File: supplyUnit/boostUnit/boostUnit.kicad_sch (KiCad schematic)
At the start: 25 parts, among them J1 Conn_02x03_Counter_Clockwise, J2 Conn_02x03_Counter_Clockwise

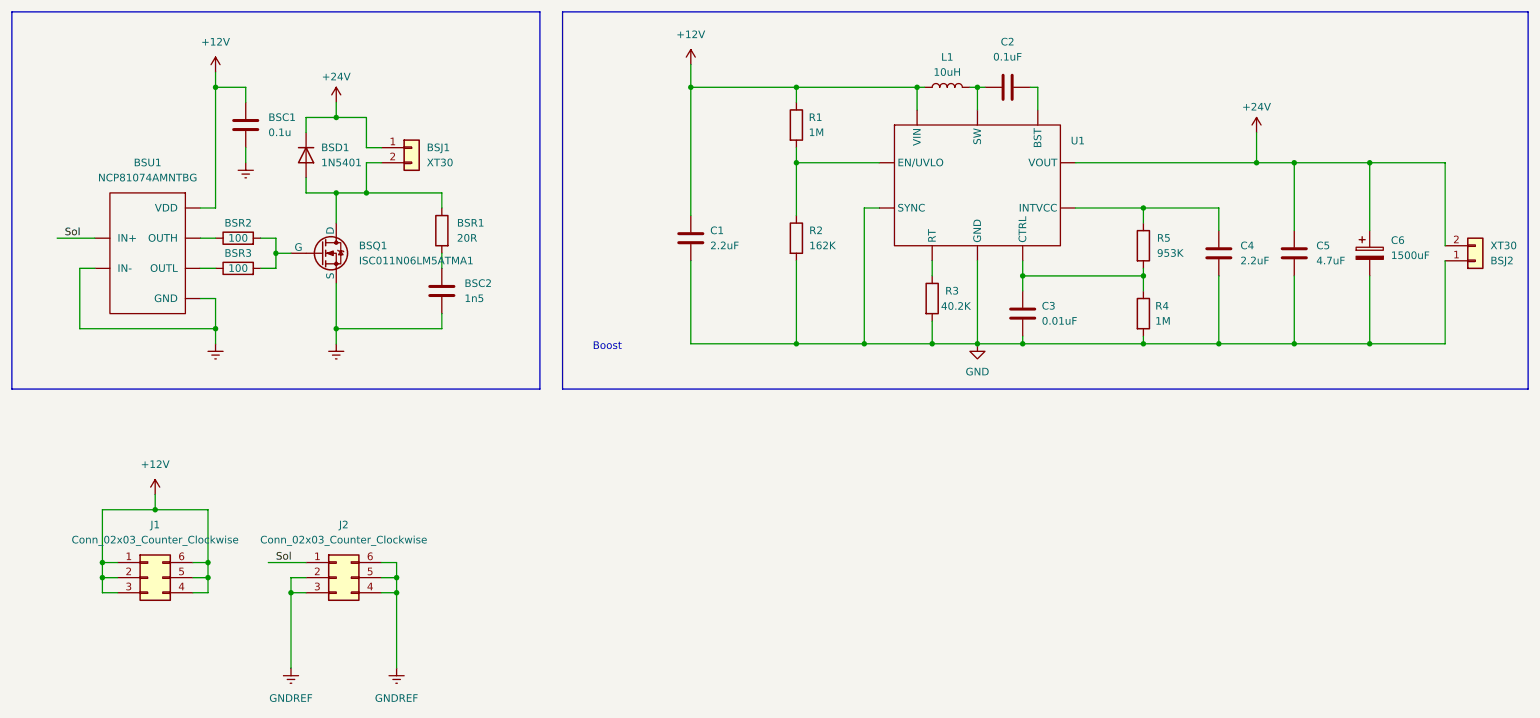
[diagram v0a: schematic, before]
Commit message: Revert
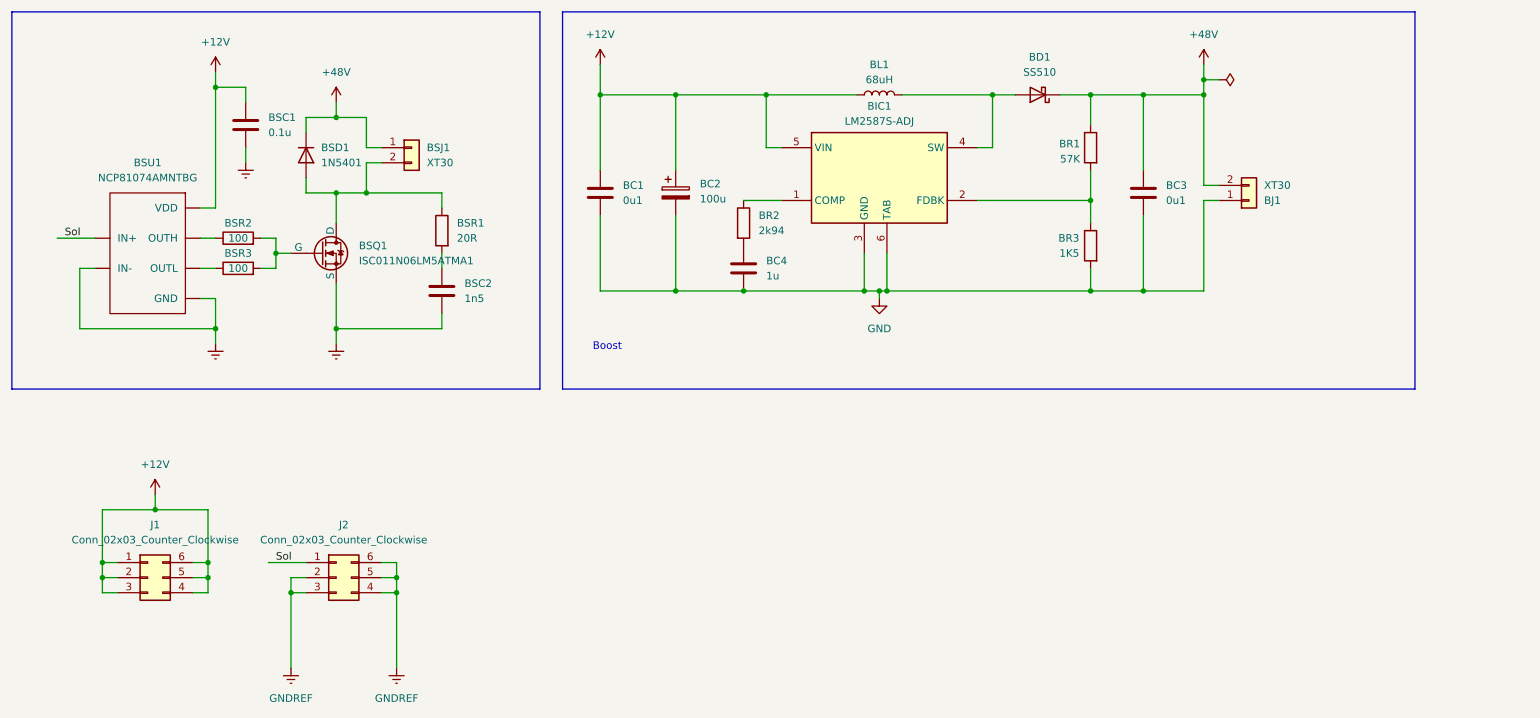
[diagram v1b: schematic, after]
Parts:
- removed BSJ2: XT30, Library:AMASS_XT30PW-F_1x02_P2.50mm_Horizontal, symbol Connector_Generic:Conn_01x02
- removed C1, C4: 2.2uF, Boost:cap0805, symbol Device:C
- removed C2: 0.1uF, Boost:cap0402, symbol Device:C
- removed C3: 0.01uF, Boost:cap0402, symbol Device:C
- removed C5: 4.7uF, Boost:res0805, symbol Device:C
- removed C6: 1500uF, Boost:CP_Radial_D16.0mm_P7.50mm, symbol Device:C_Polarized
- removed L1: 10uH, Boost:res0805, symbol Device:L
- removed R1, R4: 1M, Boost:res0402, symbol Device:R
- removed R2: 162K, Boost:res0402, symbol Device:R
- removed R3: 40.2K, Boost:res0402, symbol Device:R
- removed R5: 953K, Boost:res0402, symbol Device:R
- removed U1: ~, Boost:LT8338, symbol boostUnit:LT8338
- added BC1, BC3: 0u1, Library:cap0603, symbol Device:C
- added BC2: 100u, Capacitor_SMD:CP_Elec_8x6.5, symbol Device:C_Polarized
- added BC4: 1u, Library:cap0603, symbol Device:C
- added BD1: SS510, Library:SMA (DO-214AC), symbol Device:D_Schottky
- added BIC1: LM2587S-ADJ, Library:TO170P1435X465-6N, symbol LM2587S-ADJ_NOPB:LM2587S-ADJ_NOPB
- added BJ1: XT30, Library:AMASS_XT30PW-F_1x02_P2.50mm_Horizontal, symbol Connector_Generic:Conn_01x02
- added BL1: 68uH, Library:1040 One Piece Inductor, symbol Device:L
- added BR1: 57K, Library:res0603, symbol Device:R
- added BR2: 2k94, Library:res0603, symbol Device:R
- added BR3: 1K5, Library:res0603, symbol Device:R
- BSC1, BSR1, BSR2, BSR3: footprint Boost:res0603 -> Library:res0603
- BSC2: footprint Boost:cap0603 -> Library:cap0603
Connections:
- net +12V: now also BC1.1, BC2.1, BIC1.5 (VIN), BL1.1
- net GND: now also BC1.2, BC2.2, BC3.2, BC4.2, BIC1.3 (GND), BIC1.6 (TAB), BJ1.1 (Pin_1), BR3.2
- net +24V renamed +48V
- net +48V: now also BC3.1, BD1.1 (K), BJ1.2 (Pin_2), BR1.1
- new net: BIC1.1 (COMP), BR2.1
- new net: BIC1.2 (FDBK), BR1.2, BR3.1
- new net: BD1.2 (A), BIC1.4 (SW), BL1.2
- new net: BC4.1, BR2.2
